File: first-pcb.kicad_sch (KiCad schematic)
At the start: 7 parts

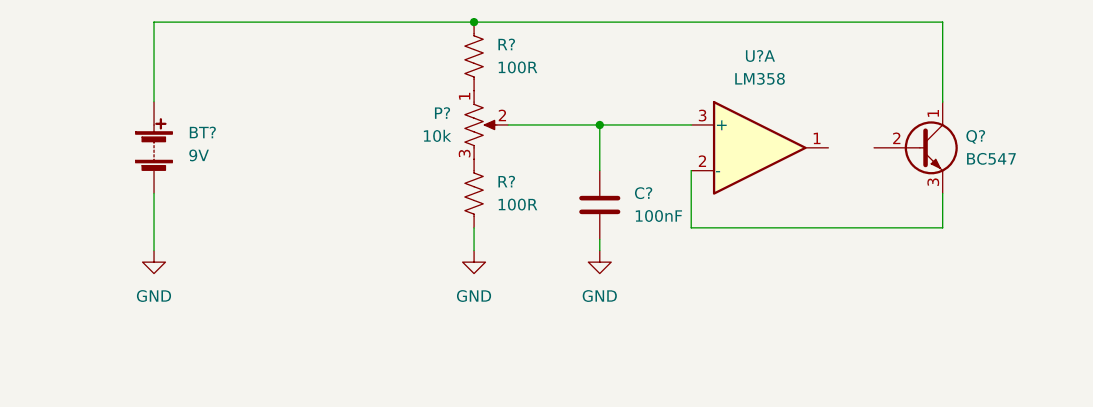
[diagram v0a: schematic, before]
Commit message: Schematic Complete
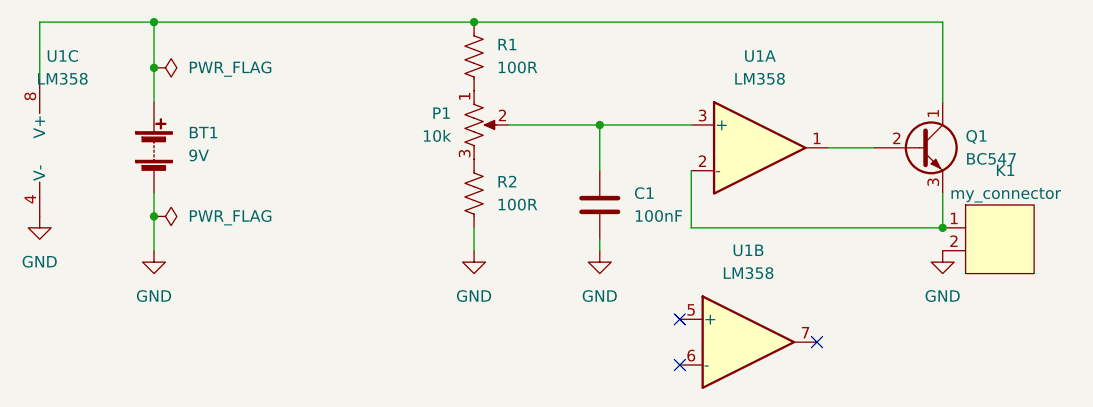
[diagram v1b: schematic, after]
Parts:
- added K1: my_connector, Connector_PinHeader_2.54mm:PinHeader_1x02_P2.54mm_Vertical, symbol my_library:my_connector
- added unit 2 of U1
- added unit 3 of U1
- BT1: renamed from BT?; footprint (none) -> Battery:BatteryHolder_Eagle_12BH611-GR
- C1: renamed from C?; footprint (none) -> Capacitor_THT:C_Disc_D3.0mm_W2.0mm_P2.50mm
- P1: renamed from P?; footprint (none) -> Potentiometer_THT:Potentiometer_Alps_RK09K_Single_Vertical
- U1: renamed from U?; footprint (none) -> Package_DIP:DIP-8_W7.62mm
- gave numbers to parts that had none: 3
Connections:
- net GND: now also K1.2, U1.4 (V-)
- net at BT1.1 (+), Q1.1 (C), R1.1: now also U1.8 (V+)
- net at U1.1: now also Q1.2 (B)
- net at Q1.3 (E), U1.2 (-): now also K1.1
- no-connect marks 0 -> 3
